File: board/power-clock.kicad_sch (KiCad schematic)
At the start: 15 parts, among them J13 Barrel_Jack_Switch, SW1 RESET, Y4 SYSCLK

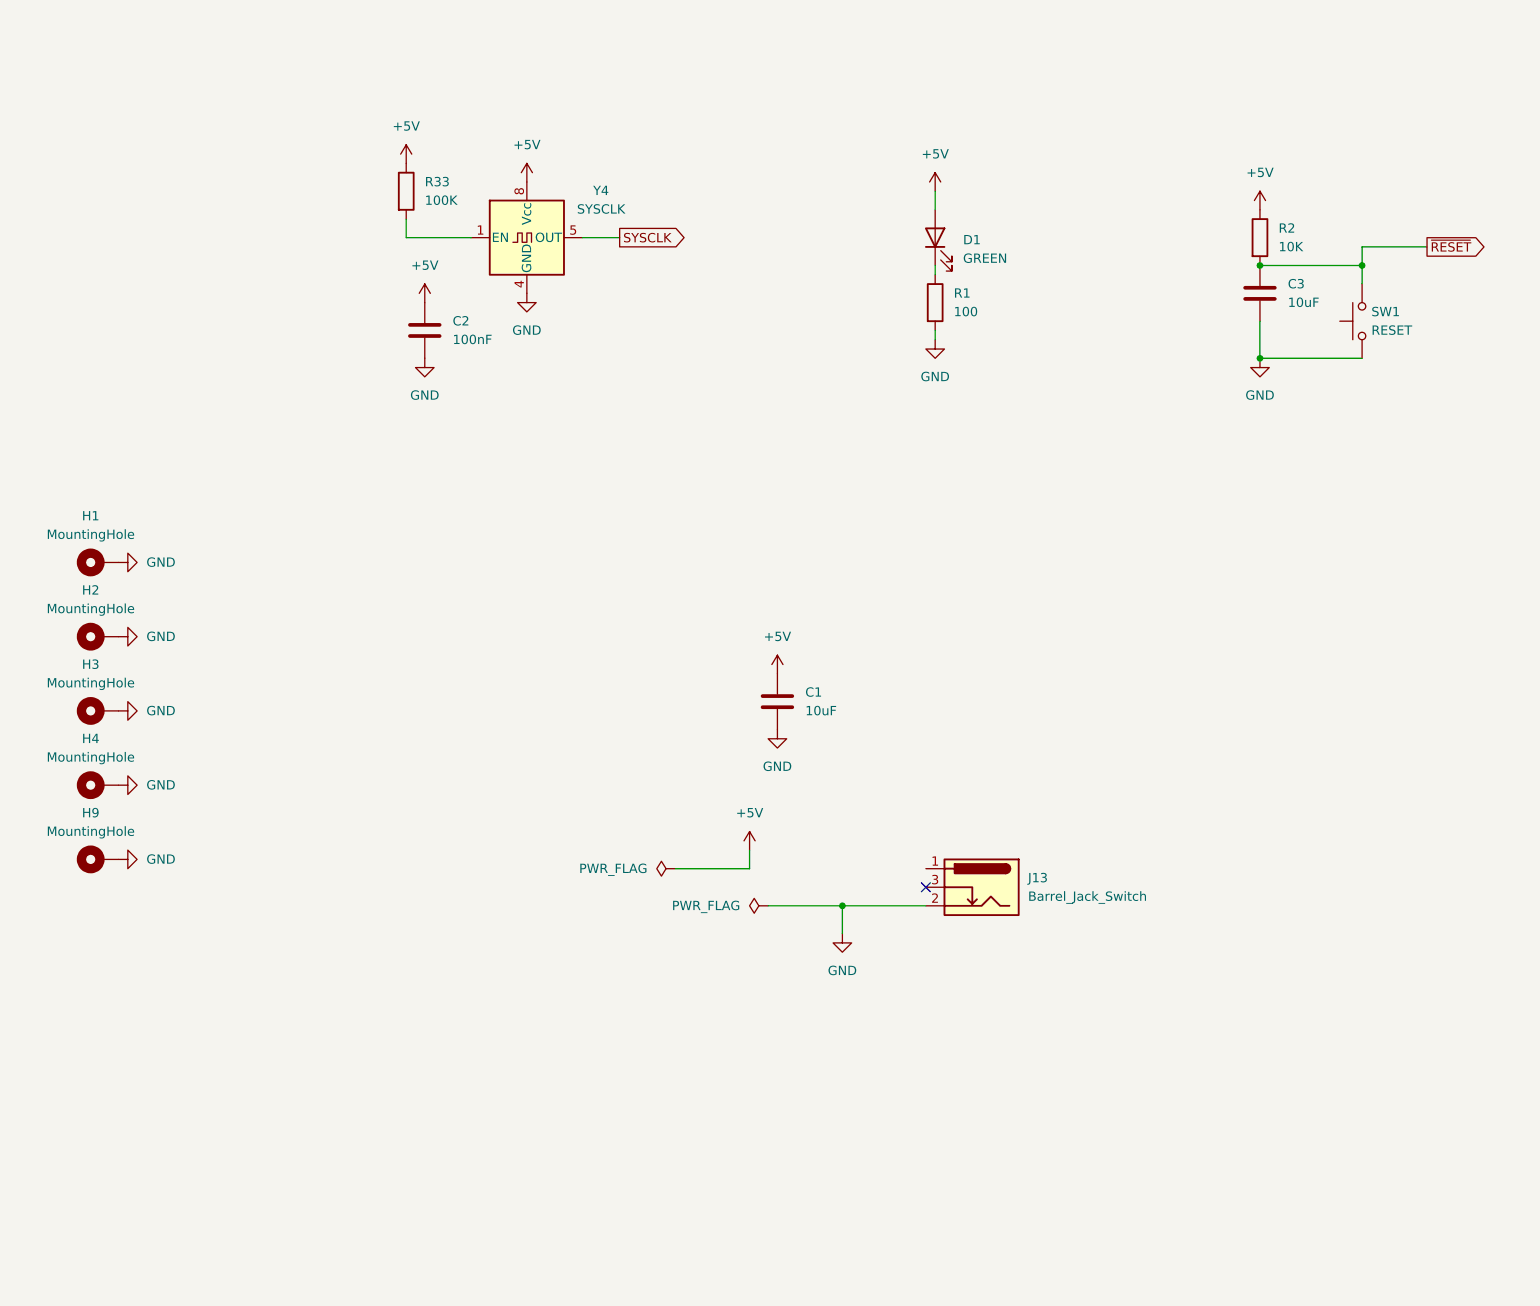
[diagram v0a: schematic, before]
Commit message: checkpoint
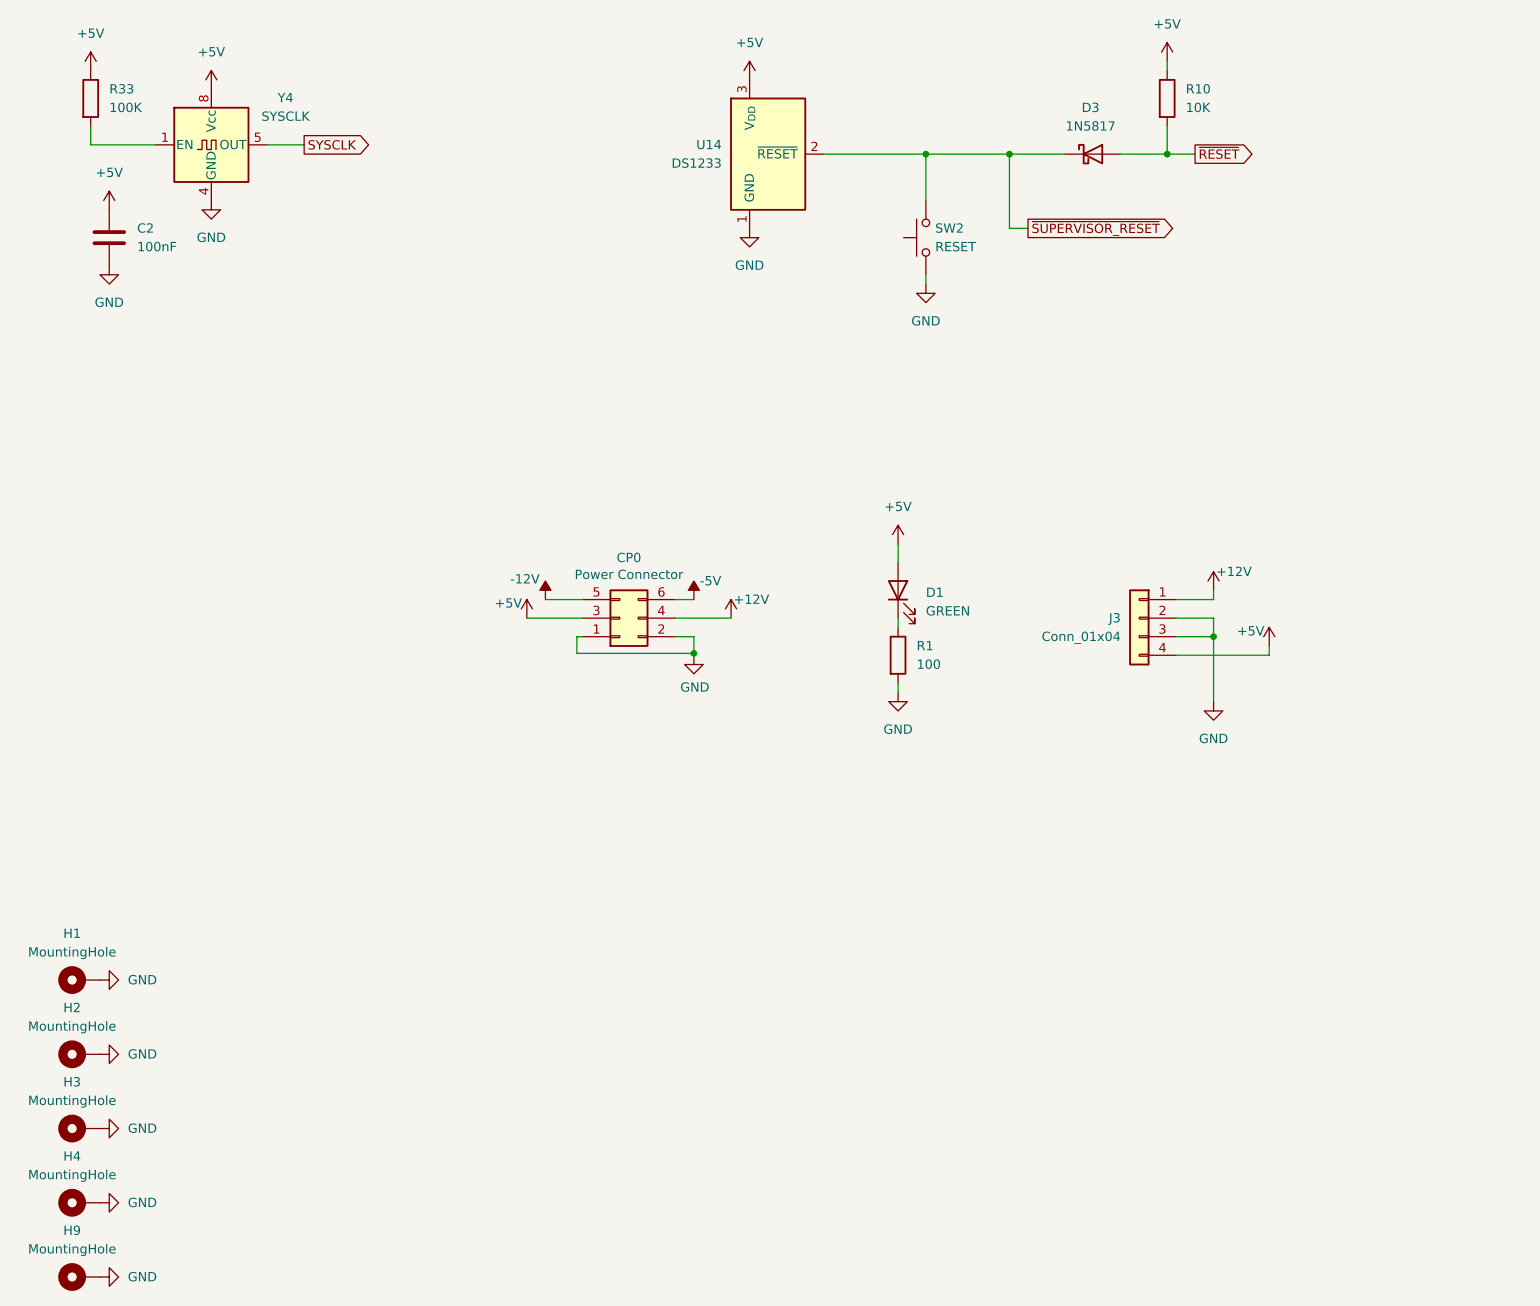
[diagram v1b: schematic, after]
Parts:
- removed C1, C3: 10uF, Capacitor_THT:CP_Radial_D5.0mm_P2.50mm, symbol Device:C
- removed J13: Barrel_Jack_Switch, symbol Connector:Barrel_Jack_Switch
- removed R2: 10K, Resistor_THT:R_Axial_DIN0207_L6.3mm_D2.5mm_P10.16mm_Horizontal, symbol Device:R
- removed SW1: RESET, Button_Switch_THT:SW_TH_Tactile_Omron_B3F-106x, symbol Switch:SW_Push
- added CP0: Power Connector, Apple-II:POWER, symbol Connector_Generic:Conn_02x03_Odd_Even
- added D3: 1N5817, Diode_THT:D_DO-41_SOD81_P10.16mm_Horizontal, symbol Diode:1N5817
- added J3: Conn_01x04, symbol Connector_Generic:Conn_01x04
- added R10: 10K, Resistor_THT:R_Axial_DIN0207_L6.3mm_D2.5mm_P10.16mm_Horizontal, symbol Device:R
- added SW2: RESET, Button_Switch_THT:SW_TH_Tactile_Omron_B3F-106x, symbol Switch:SW_Push
- added U14: DS1233, symbol Power_Supervisor:TCM809
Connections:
- net +5V: now also CP0.3 (Pin_3), J3.4 (Pin_4), R10.1, U14.3 (V_{DD})
- net GND: now also CP0.1 (Pin_1), CP0.2 (Pin_2), J3.2 (Pin_2), J3.3 (Pin_3), SW2.1, U14.1 (GND)
- net ~{RESET}: now also D3.2 (A), R10.2
- new net +12V: CP0.4 (Pin_4), J3.1 (Pin_1)
- new net -12V: CP0.5 (Pin_5)
- new net -5V: CP0.6 (Pin_6)
- new net ~{SUPERVISOR_RESET}: D3.1 (K), SW2.2, U14.2 (~{RESET})
- no-connect marks 1 -> 0
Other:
- moved on the sheet: C2, D1, H1, H2, H3, H4, H9, R1, R33, Y4
